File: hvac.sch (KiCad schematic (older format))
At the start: 53 parts, among them IC1 ATMEGA328P-A, J1 PROGRAMMING HEADER, J2 SERIAL PORT, J3 POWER_INPUT, M1 FIDUCIAL, M2 FIDUCIAL, M3 FIDUCIAL, SW1 SPST, SW2 SPST, SW3 SPST, U1 MIC5225, U2 MOSFET_N, U3 MOSFET_N, U4 MOSFET_N

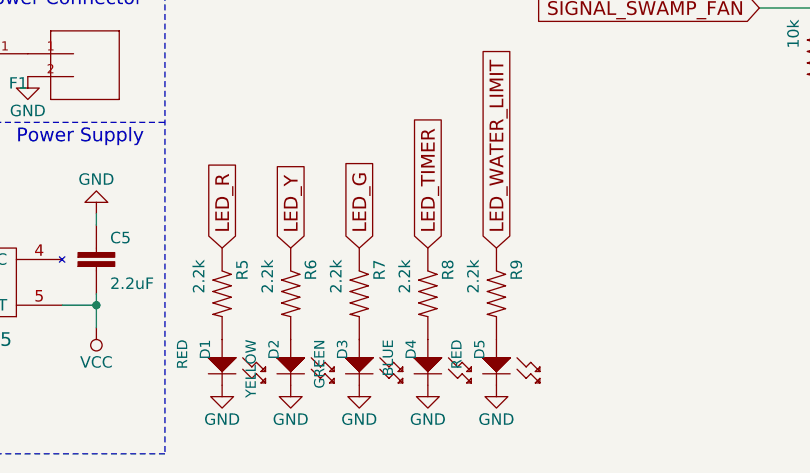
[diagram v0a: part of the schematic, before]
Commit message: Bump revision + minor changes
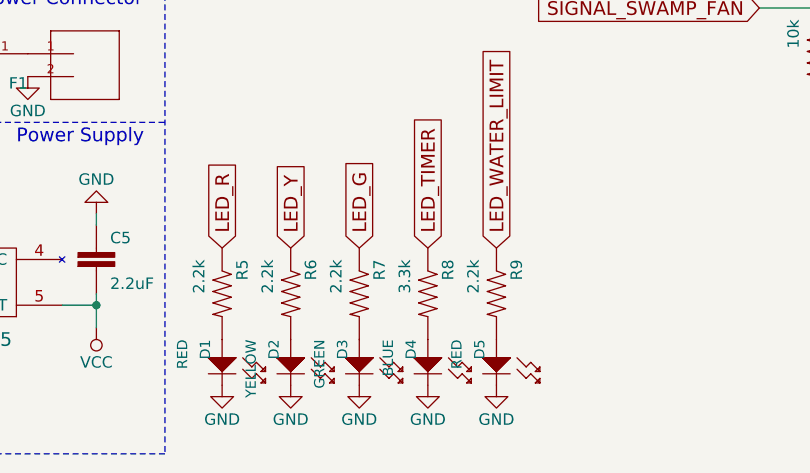
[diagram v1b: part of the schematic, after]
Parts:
- R8: value 2.2k -> 3.3k
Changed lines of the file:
@@
 P 6350 7100
 F 0 "R8" H 6200 7159 50  0000 L BNN
-F 1 "2.2k" H 6200 6970 50  0000 L BNN
+F 1 "3.3k" H 6200 6970 50  0000 L BNN
 F 2 "Resistors_SMD:R_0402" H 6380 7250 20  0001 C CNN
 F 3 "" H 6350 7100 60  0000 C CNN
